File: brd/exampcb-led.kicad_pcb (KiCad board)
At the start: 2 copper layers, 29.2 x 39.4 mm, 11 parts, among them P1 POWER, U1 LM358

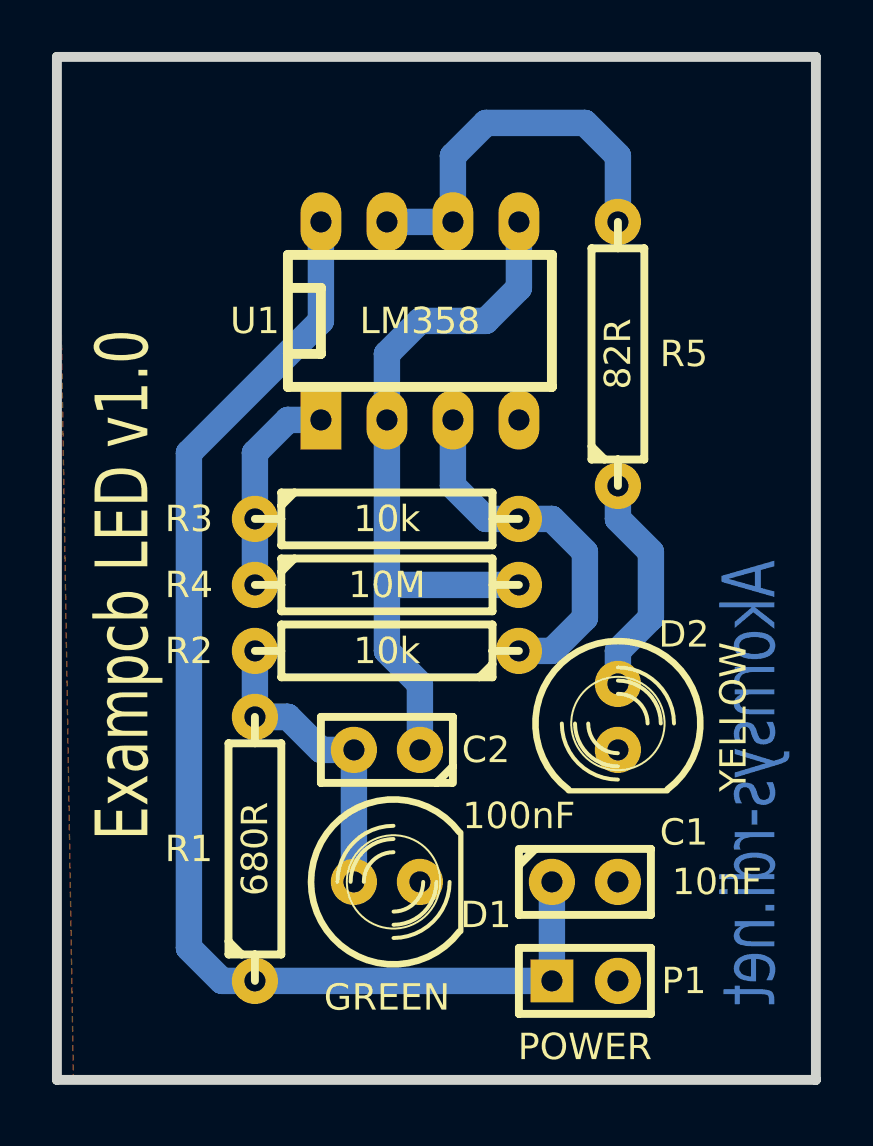
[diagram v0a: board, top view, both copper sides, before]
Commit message: new: dev: nuevo form-factor, cambio divisor y conector USB !wip
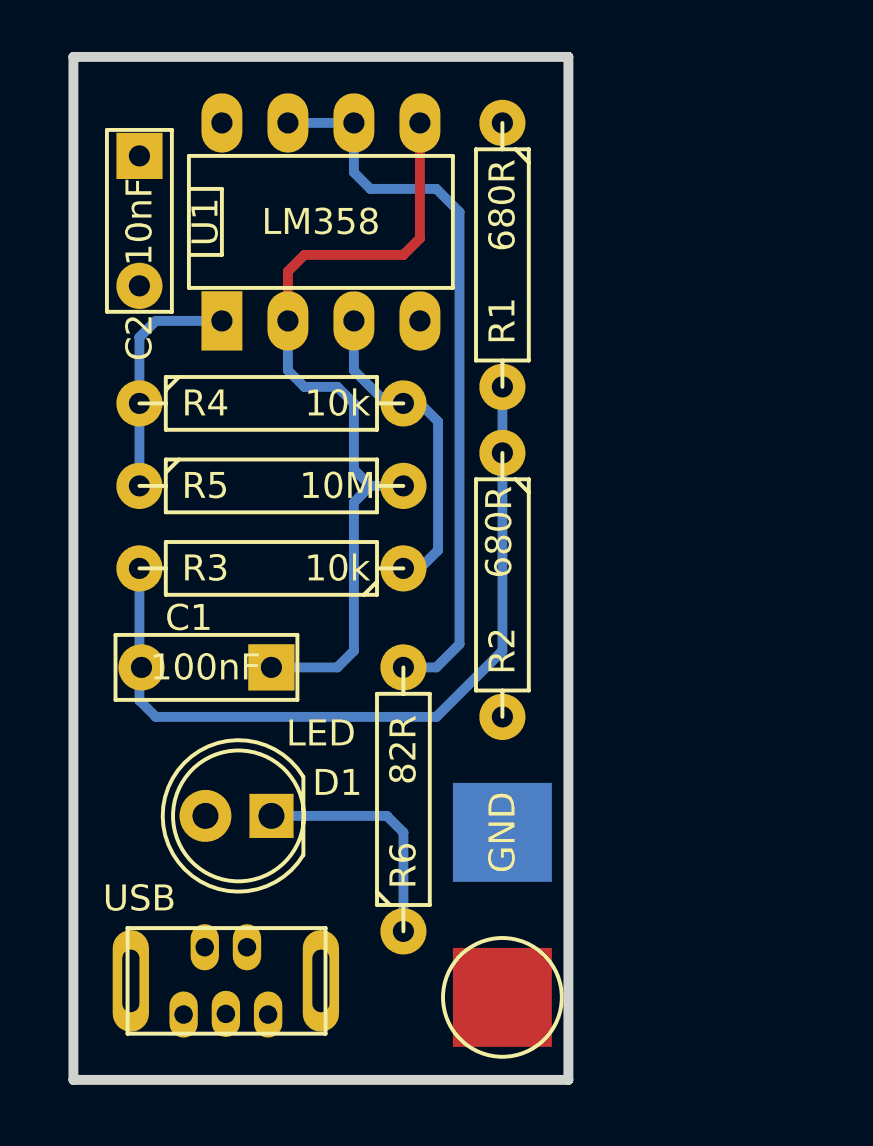
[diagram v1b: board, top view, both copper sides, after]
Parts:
- removed D2: YELLOW, LED-5MM
- removed P1: POWER, SIL-2
- added J1: USB, asrdi-conn:UE25-BEx5-10x, F.Cu at (133.7, 116.8)
- added J2: 5V, Connect:1pin, F.Cu at (148.0, 117.5)
- added J3: GND, Connect:1pin, B.Cu at (148.0, 111.1)
- added R6: 82R, Discret:R4-LARGE_PADS, F.Cu at (144.1, 109.9)
- added REF**: Symbol_OSHW-Logo_SilkScreen, Symbols:Symbol_OSHW-Logo_SilkScreen, B.Cu at (146.7, 99.7)
- C1: value 10nF -> 100nF; footprint C1 -> Capacitors_ThroughHole:C_Rect_L7_W2.5_P5
- C2: value 100nF -> 10nF; footprint C1 -> Capacitors_ThroughHole:C_Rect_L7_W2.5_P5
- D1: value GREEN -> LED; footprint LED-5MM -> LEDs:LED-5MM
- R1, R3: footprint R4 -> Discret:R4-LARGE_PADS
- R2: value 10k -> 680R; footprint R4 -> Discret:R4-LARGE_PADS
- R4: value 10M -> 10k; footprint R4 -> Discret:R4-LARGE_PADS
- R5: value 82R -> 10M; footprint R4 -> Discret:R4-LARGE_PADS
- U1: footprint DIP-8__300_ELL -> Housings_DIP:DIP-8__300_ELL
- moved R1 24.8 mm to (148.0, 88.9), turned to 270 degrees
- moved C2 24.8 mm to (134.0, 85.1), turned to 270 degrees
- moved C1 14.6 mm to (139.1, 104.8), turned to 180 degrees
- moved R5 14.3 mm to (139.1, 97.8), turned to 0 degrees
- moved R4 8.28 mm to (139.1, 94.6)
- moved U1 5.39 mm to (141.0, 87.6)
- moved R2 5.12 mm to (148.0, 101.6), turned to 270 degrees
- moved D1 5.12 mm to (139.1, 110.5), turned to 180 degrees
- moved R3 4.84 mm to (139.1, 101.0), turned to 180 degrees
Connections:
- C1 pad 1: VCC -> Net-(C1-Pad1)
- C1 pad 2: GND -> Net-(C1-Pad2)
- C2 pad 1: N-000007 -> VCC
- C2 pad 2: N-000003 -> GND
- D1 pad 1: N-000003 -> Net-(D1-Pad1)
- R1 pad 2: N-000003 -> Net-(C1-Pad2)
- R2 pad 1: N-000004 -> Net-(C1-Pad2)
- R2 pad 2: N-000003 -> GND
- R3 pad 1: N-000006 -> Net-(R3-Pad1)
- R3 pad 2: N-000004 -> Net-(C1-Pad2)
- R4 pad 1: N-000006 -> Net-(R4-Pad1)
- R4 pad 2: N-000007 -> Net-(R3-Pad1)
- R5 pad 1: N-000005 -> Net-(R4-Pad1)
- R5 pad 2: N-000001 -> Net-(C1-Pad1)
- U1 pad 1: N-000006 -> Net-(R4-Pad1)
- U1 pad 2: N-000007 -> Net-(C1-Pad1)
- U1 pad 3: N-000004 -> Net-(R3-Pad1)
- U1 pad 5: N-000007 -> Net-(C1-Pad1)
- U1 pad 6: N-000001 -> Net-(R6-Pad2)
- U1 pad 7: N-000001 -> Net-(R6-Pad2)
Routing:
- net VCC: track 48.4 -> 0.00 mm
- net Net-(C1-Pad1): track 0.00 -> 31.7 mm
- net Net-(C1-Pad2): track 0.00 -> 30.7 mm
- net N-000007: track 29.5 -> 0.00 mm
- net Net-(R6-Pad2): track 0.00 -> 28.3 mm
- net N-000001: track 15.0 -> 0.00 mm
- net N-000004: track 14.3 -> 0.00 mm
- net N-000003: track 13.2 -> 0.00 mm
- net Net-(R3-Pad1): track 0.00 -> 12.5 mm
- net Net-(R4-Pad1): track 0.00 -> 9.15 mm
- net Net-(D1-Pad1): track 0.00 -> 9.15 mm
- net N-000005: track 8.67 -> 0.00 mm
- net N-000006: track 8.15 -> 0.00 mm
- added copper zone on F.Cu, net VCC
- removed copper zone on F.Cu, net GND
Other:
- board size 29.2 x 39.4 mm -> 19.1 x 39.4 mm
- board text added: "Copyright (C) 2015 kwendenarmo https://github.com/akornsys-rdi/exampcb-led"
- board text added: "Released under GNU/GPL 3 License https://www.gnu.org/licenses/gpl.html"
- board text removed: "Akornsys-rdi.net"
